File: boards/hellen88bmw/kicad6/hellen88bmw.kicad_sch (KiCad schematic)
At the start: 267 parts, among them J1 920-462A2021Y10101, J10 Conn_01x12, J11 Conn_01x12, J12 Conn_01x12, J13 Conn_01x12, J14 VRIN1, J15 VRIN2, J16 VROUT1, J18 C165947, J2 UB-20PMFP-LC7002, J3 Micro_SD_Card, J4 Conn_01x05, J5 Conn_01x12, J6 Conn_01x12, J7 Conn_01x12, J8 Conn_01x12, J9 Conn_01x12, M1 Module-power12-0.1, M10 Module-ign8-0.1, M11 Module-mcu-0.1, M12 Module-knock-0.1, M2 Module-can-0.1, M3 Module-wbo-0.1, M4 Module-can-0.1, M5 Module-power5-0.1, M6 Module-vr-0.1, M7 Module-input-0.1, M8 Module-knock-0.1, M9 Module-output-0.1, Q1 NGD8201AN, Q2 NGD8201AN, Q3 NGD8201AN, Q4 NGD8201AN, Q5 NGD8201AN, Q6 NGD8201AN, Q7 NGD8201AN, Q8 NGD8201AN, SW1 BOOT0, SW2 RESET, U1 MPXA6115A, U2 MPX4_MAP, U3 LIS2DW12TR, U4 LPS25HB, U5 MCP6002-xSN

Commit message: Up hellen88bmw 6.07.2021
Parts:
- removed OUT_INJ1: OUT_INJ1, Connector_PinHeader_1.00mm:PinHeader_1x01_P1.00mm_Vertical, symbol Connector_Generic:Conn_01x01
- removed OUT_INJ2: OUT_INJ2, Connector_PinHeader_1.00mm:PinHeader_1x01_P1.00mm_Vertical, symbol Connector_Generic:Conn_01x01
- removed OUT_INJ3: OUT_INJ3, Connector_PinHeader_1.00mm:PinHeader_1x01_P1.00mm_Vertical, symbol Connector_Generic:Conn_01x01
- removed OUT_INJ4: OUT_INJ4, Connector_PinHeader_1.00mm:PinHeader_1x01_P1.00mm_Vertical, symbol Connector_Generic:Conn_01x01
- removed OUT_INJ5: OUT_INJ5, Connector_PinHeader_1.00mm:PinHeader_1x01_P1.00mm_Vertical, symbol Connector_Generic:Conn_01x01
- removed OUT_INJ6: OUT_INJ6, Connector_PinHeader_1.00mm:PinHeader_1x01_P1.00mm_Vertical, symbol Connector_Generic:Conn_01x01
- removed OUT_INJ7: OUT_INJ7, Connector_PinHeader_1.00mm:PinHeader_1x01_P1.00mm_Vertical, symbol Connector_Generic:Conn_01x01
- removed OUT_INJ8: OUT_INJ8, Connector_PinHeader_1.00mm:PinHeader_1x01_P1.00mm_Vertical, symbol Connector_Generic:Conn_01x01
- added J17: XH-8A, symbol Connector_Generic:Conn_01x08
- added JP2: Jumper_2_Open, rusefi_lib:SM0805_jumper, symbol Jumper:Jumper_2_Open
- added MMCU20, MMCU21, MMCU22, MMCU23, MMCU37, MMCU38, MMCU39, MMCU40, MMCU41: MMCU, Connector_PinHeader_1.00mm:PinHeader_1x01_P1.00mm_Vertical, symbol Connector_Generic:Conn_01x01
- added P1, P2, P3, P4, P5, P6: P, Connector_PinHeader_1.00mm:PinHeader_1x01_P1.00mm_Vertical, symbol Connector_Generic:Conn_01x01
- added VIN18, VIN19, VIN20, VIN21, VIN23, VIN24, VIN25, VOUT21, VOUT24, VOUT25, VOUT26, VOUT27, VOUT28, VOUT29: Pad, Connector_PinHeader_1.00mm:PinHeader_1x01_P1.00mm_Vertical, symbol hellen-one-common:Pad
- added VIN22: VIN5, Connector_PinHeader_1.00mm:PinHeader_1x01_P1.00mm_Vertical, symbol Connector_Generic:Conn_01x01
- added VOUT22, VOUT23: VOUT4, Connector_PinHeader_1.00mm:PinHeader_1x01_P1.00mm_Vertical, symbol Connector_Generic:Conn_01x01
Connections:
- net 5V_SENS1 is gone; now on net 5V_SENS2: JP59.2 (B)
- net CRANK+ is gone; now on net IN_CRANK+: D3.2 (A), JP16.2 (B)
- net CRANK- is gone; now on net IN_CRANK-: D8.2 (A), JP43.2 (B)
- net D3 is gone; now on an unnamed net: M11.S5 (IN_D3)
- net MAP_AV1 is gone; now on net IN_MAP2: U2.1 (VOUT)
- net CRANK: no longer D7.2 (A)
- net GND: now also J17.1 (Pin_1), J17.2 (Pin_2), P1.1 (Pin_1)
- net INJ1: no longer JP33.2 (B)
- net INJ2: no longer JP32.2 (B)
- net INJ3: no longer JP31.2 (B)
- net INJ4: no longer JP5.2 (B)
- net INJ5: no longer JP3.2 (B)
- net INJ6: no longer JP4.2 (B)
- net INJ7: no longer JP7.2 (B)
- net INJ8: no longer JP35.2 (B)
- net IN_CRANK: now also D7.2 (A)
- net IN_KNOCK1: no longer M7.N22 (KNOCK)
- net IN_KNOCK2: no longer M7.N24 (SENS3)
- net IN_VIGN: now also JP2.2 (B)
- net LSU_CALIBR_RES: now also J17.5 (Pin_5), P3.1 (Pin_1)
- net LSU_HEAT-: now also J17.3 (Pin_3), J17.4 (Pin_4), P2.1 (Pin_1)
- net LSU_PUMP_I: now also J17.6 (Pin_6), P4.1 (Pin_1)
- net LSU_SENSOR_U: now also J17.8 (Pin_8), P6.1 (Pin_1)
- net LSU_SENSOR_U/PUMP_I: now also J17.7 (Pin_7), P5.1 (Pin_1)
- net OUT_INJ1: now also JP33.2 (B)
- net OUT_INJ2: now also JP32.2 (B)
- net OUT_INJ3: now also JP31.2 (B)
- net OUT_INJ4: now also JP5.2 (B)
- net OUT_INJ5: now also JP3.2 (B)
- net OUT_INJ6: now also JP4.2 (B)
- net OUT_INJ7: now also JP7.2 (B)
- net OUT_INJ8: now also JP35.2 (B)
- net V12_RAW: now also JP2.1 (A)
- net at M7.S17 (IN_AUX1): now also VIN23.1 (Pin_1)
- net at M7.S21 (IN_AUX4): now also VIN25.1 (Pin_1)
- net at MMCU35.1 (Pin_1): no longer M11.S10 (IN_SENS3)
- net at MMCU16.1 (Pin_1): now also M11.E14 (OUT_PWM1); no longer M11.S27 (IN_AUX4)
- net at M11.E12 (OUT_IO7): now also MMCU39.1 (Pin_1)
- net at M7.N7 (AUX4): now also VIN22.1 (Pin_1)
- net BARO_AV5 renamed BARO
- net BARO: now also M11.S27 (IN_AUX4)
- net CE: no longer names the net of M9.W25 (LOW4_DIODE)
- net CE: now also VOUT26.1 (Pin_1); no longer M11.E22 (OUT_IO11)
- net COIL_A1: no longer names the net of M9.W33 (SOLENOID_A1)
- net COIL_A1: now also VOUT24.1 (Pin_1); no longer M11.E14 (OUT_PWM1)
- net COIL_A2: no longer names the net of M11.E15 (OUT_PWM2)
- net COIL_A2: now also MMCU20.1 (Pin_1); no longer M9.W32 (SOLENOID_A2)
- net D1: no longer names the net of M11.S3 (IN_D1)
- net D1: now also MMCU22.1 (Pin_1)
- net D2: no longer names the net of M11.S4 (IN_D2)
- net D2: now also MMCU23.1 (Pin_1)
- net D4: no longer names the net of M11.S6 (IN_D4)
- net D4: now also MMCU37.1 (Pin_1)
- net IN_A1: no longer names the net of M7.S25 (IN_O2S2), VIN1.1 (Pin_1)
- net IN_A2: no longer names the net of M7.S19 (IN_MAP3), VIN2.1 (Pin_1)
- net IN_A3: no longer names the net of M7.S20 (IN_AUX3)
- net IN_A3: now also VIN24.1 (Pin_1); no longer VIN3.1 (Pin_1)
- net IN_A4: no longer names the net of M7.S22 (IN_RES3), VIN4.1 (Pin_1)
- net IN_AFR: no longer names the net of M7.S9 (IN_O2S)
- net IN_AFR: now also VIN18.1 (Pin_1)
- net IN_PPS1: no longer names the net of M7.S24 (IN_PPS)
- net IN_PPS1: now also VIN21.1 (Pin_1)
- net IN_PPS2: no longer names the net of M7.S18 (IN_AUX2)
- net IN_PPS2: now also VIN3.1 (Pin_1)
- net IN_RES1: no longer names the net of M7.S23 (IN_RES1)
- net IN_RES1: now also VIN19.1 (Pin_1)
- net IN_RES2: no longer names the net of M7.S26 (IN_RES2)
- net IN_RES2: now also VIN20.1 (Pin_1)
- net KNOCK1 renamed INK1
- net INK1: now also M7.N22 (KNOCK)
- net OUT1: no longer names the net of M11.E7 (OUT_IO2)
- net OUT1: now also MMCU41.1 (Pin_1); no longer M9.W39 (LOW5_HIGH1)
- net OUT2: no longer names the net of M11.E9 (OUT_IO4)
- net OUT2: now also MMCU38.1 (Pin_1); no longer M9.W37 (LOW6_HIGH2)
- net OUT3: no longer names the net of M9.W21 (LOW8)
- net OUT3: now also VOUT29.1 (Pin_1); no longer M11.E28 (OUT_PWM8)
- net OUT_CE: no longer names the net of M9.W3 (OUT_LOW4_DIODE)
- net OUT_CE: now also VOUT21.1 (Pin_1)
- net OUT_COIL_A1: no longer names the net of M9.S1 (OUT_SOLENOID_A1)
- net OUT_COIL_A1: now also VOUT22.1 (Pin_1)
- net OUT_COIL_A2: no longer names the net of M9.S2 (OUT_SOLENOID_A2)
- net OUT_COIL_A2: now also VOUT23.1 (Pin_1)
- new net: M11.E22 (OUT_IO11), MMCU40.1 (Pin_1)
- new net: M11.E28 (OUT_PWM8), MMCU21.1 (Pin_1)
- new net: M9.W32 (SOLENOID_A2), VOUT25.1 (Pin_1)
- new net: M9.W37 (LOW6_HIGH2), VOUT28.1 (Pin_1)
- new net: M9.W39 (LOW5_HIGH1), VOUT27.1 (Pin_1)
- new net INK2: M11.S10 (IN_SENS3), M7.N24 (SENS3)
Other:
- moved on the sheet: *ref1A, *ref1B, *ref1C, C1, C2, C3, C4, C5, C6, C7, C8, D1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

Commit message: Up issue 26.28.29
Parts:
- removed unit 2 of M9
- added unit 3 of M9
- added unit 2 of M9
- M1: value Module-power12-0.1 -> Module-power12-0.2; footprint power12:power12 -> hellen-one-power12-0.2:power12; symbol hellen-one-power12-0.1:Module-power12-0.1 -> hellen-one-power12-0.2:Module-power12-0.2
- M10: footprint ign8:ign8 -> hellen-one-ign8-0.1:ign8
- M11: value Module-mcu-0.1 -> Module-mcu-0.4; footprint mcu:mcu -> hellen-one-mcu-0.4:mcu; symbol hellen-one-mcu-0.1:Module-mcu-0.1 -> hellen-one-mcu-000.4:Module-mcu-0.4
- M12, M8: footprint knock:knock -> hellen-one-knock-0.1:knock
- M2, M4: footprint can:can -> hellen-one-can-0.1:can
- M3: value Module-wbo-0.1 -> Module-wbo-0.2; footprint wbo:wbo -> hellen-one-wbo-0.2:wbo; symbol hellen-one-wbo-0.1:Module-wbo-0.1 -> hellen-one-wbo-0.2:Module-wbo-0.2
- M5: footprint power5:power5 -> hellen-one-power5-0.1:power5; symbol hellen-one-power5-0.1:Module-power5-0.1 -> hellen-one-power5-0.2:Module-power5-0.1
- M6: footprint vr:vr -> hellen-one-vr-0.1:vr
- M7: footprint input:input -> hellen-one-input-0.1:input
- M9: value Module-output-0.1 -> Module-output-0.2; footprint output:output -> hellen-one-output-0.2:output; symbol hellen-one-output-0.1:Module-output-0.1 -> hellen-one-output-0.2:Module-output-0.2
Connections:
- net FUEL_CONSUM: now also M11.E18 (OUT_PWM6), M9.W22 (PP2); no longer M11.E19 (OUT_PWM6)
- net GND: now also M11.S32 (GNDA), M3.J_GND1 (PULL_DOWN1), M3.J_GND2 (PULL_DOWN2)
- net GNDA: no longer M11.S32 (GNDA)
- net IDLE: now also M11.E17 (OUT_PWM5), M9.W21 (LOW1); no longer M11.E18 (OUT_PWM5)
- net INJ1: now also M9.W24 (INJ1)
- net INJ2: now also M9.W23 (INJ2)
- net INJ3: now also M9.W20 (INJ3)
- net INJ4: now also M9.W19 (INJ4)
- net INJ5: now also M9.W18 (INJ5)
- net INJ6: now also M9.W17 (INJ6)
- net INJ7: now also M9.W16 (INJ7)
- net INJ8: now also M9.W15 (INJ8)
- net MAIN_RELAY: now also M9.W40 (LOW5_MAIN)
- net OUT_FUEL_CONSUM: now also M9.S6 (OUT_PP2)
- net OUT_IDLE: now also M9.S8 (OUT_LOW1)
- net OUT_INJ1: now also M9.S18 (OUT_INJ1)
- net OUT_INJ2: now also M9.S16 (OUT_INJ2)
- net OUT_INJ3: now also M9.S17 (OUT_INJ3)
- net OUT_INJ4: now also M9.W7 (OUT_INJ4)
- net OUT_INJ5: now also M9.W10 (OUT_INJ5)
- net OUT_INJ6: now also M9.S15 (OUT_INJ6)
- net OUT_INJ7: now also M9.W12 (OUT_INJ7)
- net OUT_INJ8: now also M9.W11 (OUT_INJ8)
- net OUT_MAIN: now also M11.E8 (OUT_IO1), M9.W13 (OUT_LOW5_MAIN); no longer M11.E6 (OUT_IO1)
- net OUT_PUMP: now also M9.W2 (OUT_LOW10)
- net OUT_TACH: now also M9.W6 (OUT_PP1)
- net PUMP: now also M11.E6 (OUT_IO3), M9.W26 (LOW10); no longer M11.E8 (OUT_IO3)
- net TACH: now also M11.E19 (OUT_PWM7), M9.W28 (PP1); no longer M11.E27 (OUT_PWM7)
- net at VOUT13.1 (Pin_1): now also M9.W35 (LOW11)
- net at MMCU41.1 (Pin_1): now also M11.E12 (OUT_IO2); no longer M11.E7 (OUT_IO2)
- net at VOUT5.1 (Pin_1): now also M9.S9 (OUT_HIGH2)
- net at MMCU15.1 (Pin_1): now also M11.E16 (OUT_PWM4); no longer M11.E17 (OUT_PWM4)
- net at VOUT2.1 (Pin_1): now also M9.S12 (OUT_LOW8_PULLUP)
- net at MMCU27.1 (Pin_1): now also M11.N15 (IO4); no longer M11.N15 (IO4)
- net at VOUT11.1 (Pin_1): now also M9.W38 (LOW3_DUAL)
- net at VOUT18.1 (Pin_1): now also M9.S13 (OUT_LOW12)
- net at VOUT16.1 (Pin_1): now also M9.S10 (OUT_LOW11)
- net at MMCU28.1 (Pin_1): now also M11.E9 (OUT_IO6); no longer M11.E11 (OUT_IO6)
- net at VOUT24.1 (Pin_1): now also M9.W37 (LOW8_HIGH2)
- net at MMCU26.1 (Pin_1): now also M11.N14 (IO3); no longer M11.N14 (IO3)
- net at VOUT29.1 (Pin_1): now also M9.W25 (LOW6_DIODE)
- net at VOUT7.1 (Pin_1): now also M9.W34 (LOW4_DUAL)
- net at VOUT3.1 (Pin_1): now also M9.W4 (OUT_LOW4_DUAL)
- net at VOUT26.1 (Pin_1): now also M9.W33 (SOLENOID_A1)
- net at MMCU14.1 (Pin_1): now also M11.E15 (OUT_PWM3); no longer M11.E16 (OUT_PWM3)
- net at MMCU40.1 (Pin_1): now also M11.E20 (OUT_IO11); no longer M11.E22 (OUT_IO11)
- net at VOUT22.1 (Pin_1): now also M9.S1 (OUT_SOLENOID_A1)
- net at VOUT4.1 (Pin_1): now also M9.W8 (OUT_HIGH1)
- net at M11.E10 (OUT_IO10): now also MMCU18.1 (Pin_1); no longer MMCU19.1 (Pin_1)
- net at MMCU39.1 (Pin_1): now also M11.E21 (OUT_IO7); no longer M11.E12 (OUT_IO7)
- net at M11.E13 (OUT_IO12): now also MMCU31.1 (Pin_1); no longer MMCU29.1 (Pin_1)
- net at M11.E14 (OUT_PWM2): now also MMCU20.1 (Pin_1); no longer MMCU16.1 (Pin_1)
- net at MMCU30.1 (Pin_1): now also M11.E11 (OUT_IO9); no longer M11.E20 (OUT_IO9)
- net at M11.E23 (OUT_IO4): now also MMCU38.1 (Pin_1); no longer MMCU31.1 (Pin_1)
- net at MMCU24.1 (Pin_1): now also M11.N12 (IO1); no longer M11.N12 (IO1)
- net at MMCU25.1 (Pin_1): now also M11.N13 (IO2); no longer M11.N13 (IO2)
- net at VOUT10.1 (Pin_1): now also M9.W29 (LOW2)
- net at VOUT20.1 (Pin_1): now also M9.S7 (OUT_LOW3_DUAL)
- net at VOUT19.1 (Pin_1): now also M9.W1 (OUT_LOW2)
- net at VOUT17.1 (Pin_1): now also M9.S14 (OUT_LOW9)
- net at VOUT23.1 (Pin_1): now also M9.S2 (OUT_SOLENOID_A2)
- net at VOUT14.1 (Pin_1): now also M9.S4 (OUT_SOLENOID_B1)
- net at VOUT15.1 (Pin_1): now also M9.S5 (OUT_SOLENOID_B2)
- net at VOUT9.1 (Pin_1): now also M9.W39 (LOW7_HIGH1)
- net at VOUT8.1 (Pin_1): now also M9.W30 (SOLENOID_B2)
- net at VOUT21.1 (Pin_1): now also M9.W3 (OUT_LOW6_DIODE)
- net at VOUT12.1 (Pin_1): now also M9.W36 (LOW12)
- net at VOUT25.1 (Pin_1): now also M9.W27 (LOW9)
- net at VOUT28.1 (Pin_1): now also M9.W31 (SOLENOID_B1)
- net at VOUT27.1 (Pin_1): now also M9.W32 (SOLENOID_A2)
- net at VOUT1.1 (Pin_1): now also M9.W9 (OUT_LOW7_PULLUP)
- new net: M11.E22 (OUT_IO8), MMCU29.1 (Pin_1)
- new net: M11.E27 (OUT_PWM1), MMCU16.1 (Pin_1)
- new net: M11.E7 (OUT_IO5), MMCU19.1 (Pin_1)
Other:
- moved on the sheet: C3, D1, D10, D13, D14, D2, D24, D25, D26, D27, D28, D29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

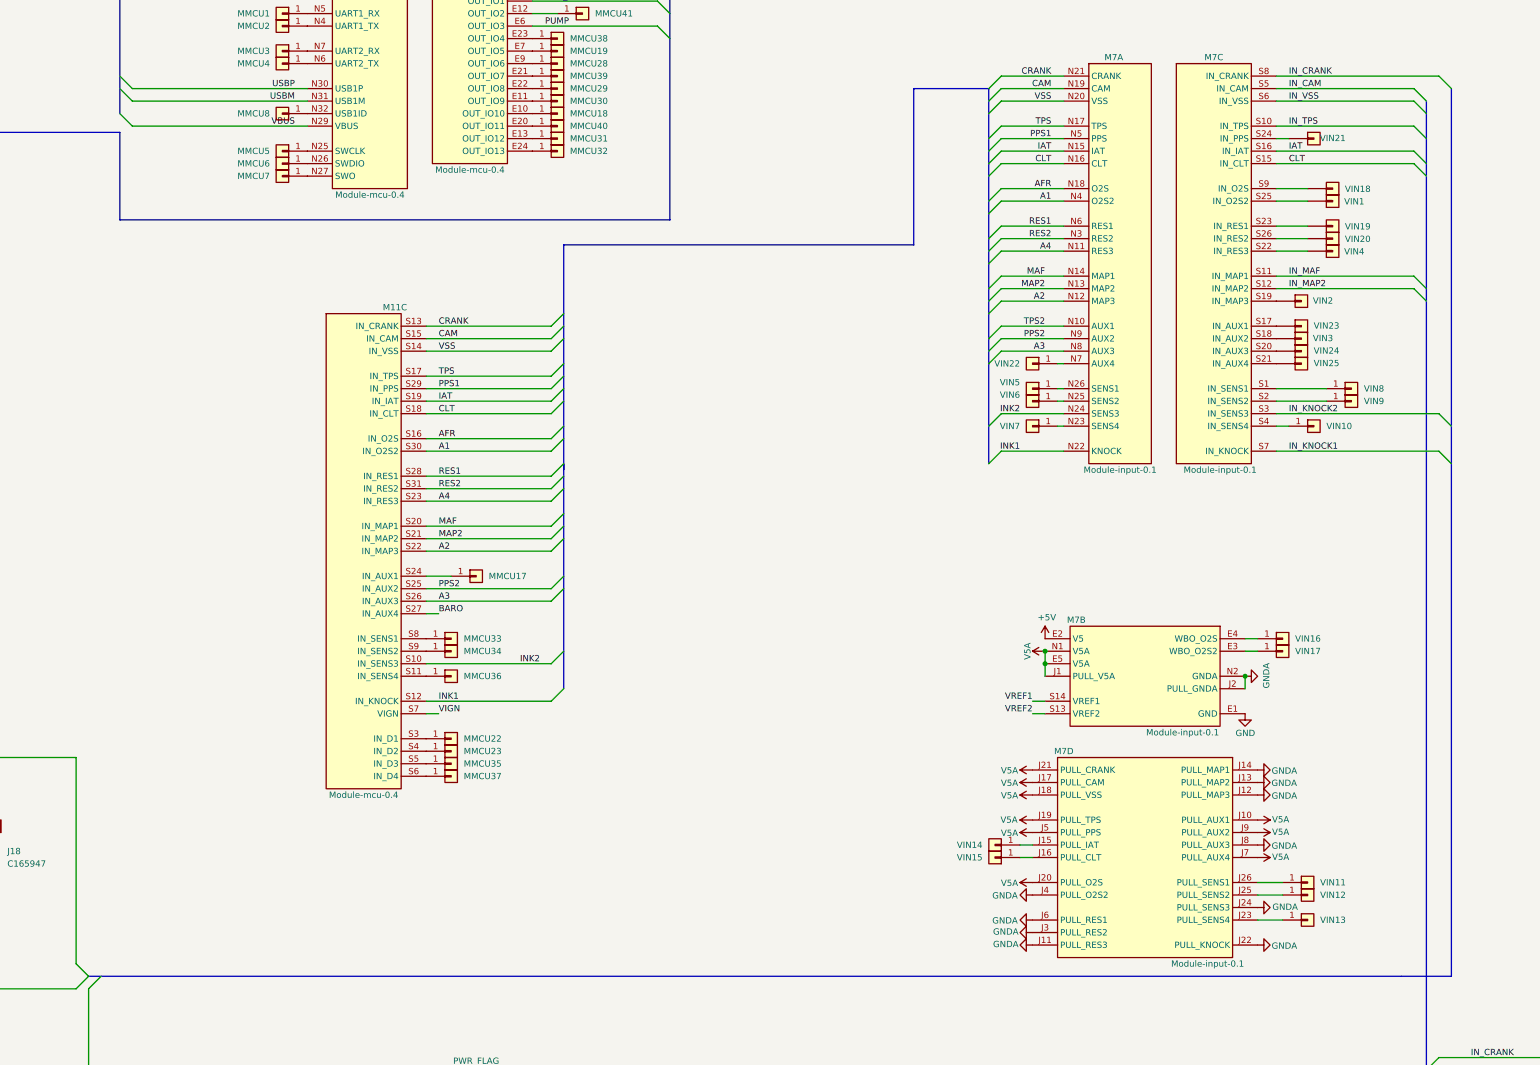
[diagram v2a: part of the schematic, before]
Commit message: Up issue 30
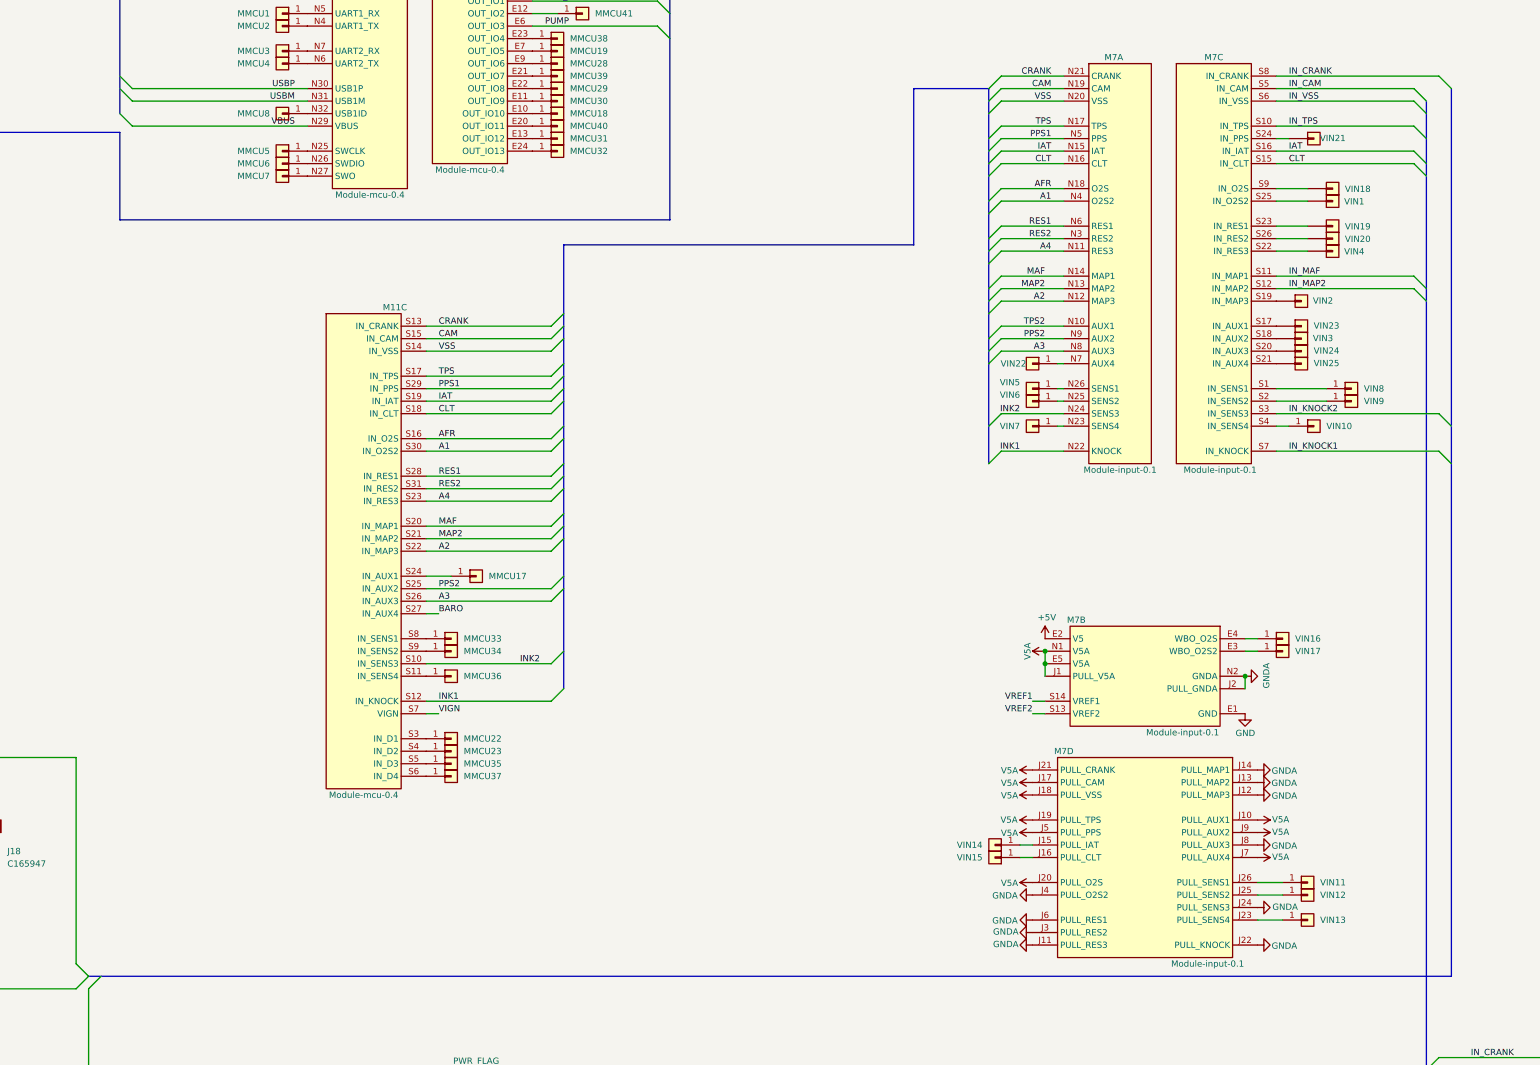
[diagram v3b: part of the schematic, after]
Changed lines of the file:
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@@
     (stroke (width 0) (type solid) (color 255 0 11 1))
   )
-  (bus (pts (xy 363.22 438.15) (xy 629.92 438.15))
+  (bus (pts (xy 363.22 438.15) (xy 640.08 438.15))
     (stroke (width 0) (type solid) (color 255 170 0 1))
   )
@@
     (stroke (width 0) (type solid) (color 153 48 255 1))
   )
-  (bus (pts (xy 459.74 289.56) (xy 459.74 335.28))
+  (bus (pts (xy 459.74 289.56) (xy 459.74 379.73))
     (stroke (width 0) (type solid) (color 255 115 103 1))
   )
@@
     (stroke (width 0) (type solid) (color 255 115 103 1))
   )
-  (bus (pts (xy 459.74 334.01) (xy 459.74 379.73))
-    (stroke (width 0) (type solid) (color 255 115 103 1))
-  )
   (bus (pts (xy 467.36 127) (xy 467.36 157.48))
     (stroke (width 0) (type solid) (color 255 129 238 1))
@@
     (stroke (width 0) (type solid) (color 132 214 255 1))
   )
-  (bus (pts (xy 640.08 257.81) (xy 640.08 334.01))
-    (stroke (width 0) (type solid) (color 255 170 0 1))
-  )
-  (bus (pts (xy 640.08 334.01) (xy 640.08 438.15))
-    (stroke (width 0) (type solid) (color 255 170 0 1))
-  )
-  (bus (pts (xy 640.08 438.15) (xy 629.92 438.15))
+  (bus (pts (xy 640.08 257.81) (xy 640.08 438.15))
     (stroke (width 0) (type solid) (color 255 170 0 1))
   )
@@
   (symbol (lib_id "Connector_Generic:Conn_01x01") (at 554.99 313.69 0) (mirror y) (unit 1)
     (in_bom yes) (on_board yes)
-    (property "Reference" "VIN22" (id 0) (at 552.45 313.69 0)
+    (property "Reference" "VIN22" (id 0) (at 553.72 313.69 0)
       (effects (font (size 1.27 1.27)) (justify left))
     )
